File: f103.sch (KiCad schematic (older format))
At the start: 211 parts, among them J1 Conn_01x04_Female, J2 Conn_01x01_Male, J3 Conn_01x01_Male, J4 Conn_01x01_Male, Q1 2N7002, SW1 Rotary_Encoder_Switch, U1 STM32F103CBTx, U2 XC6206P332MR, U3 SRV05-4, Y1 8MHz

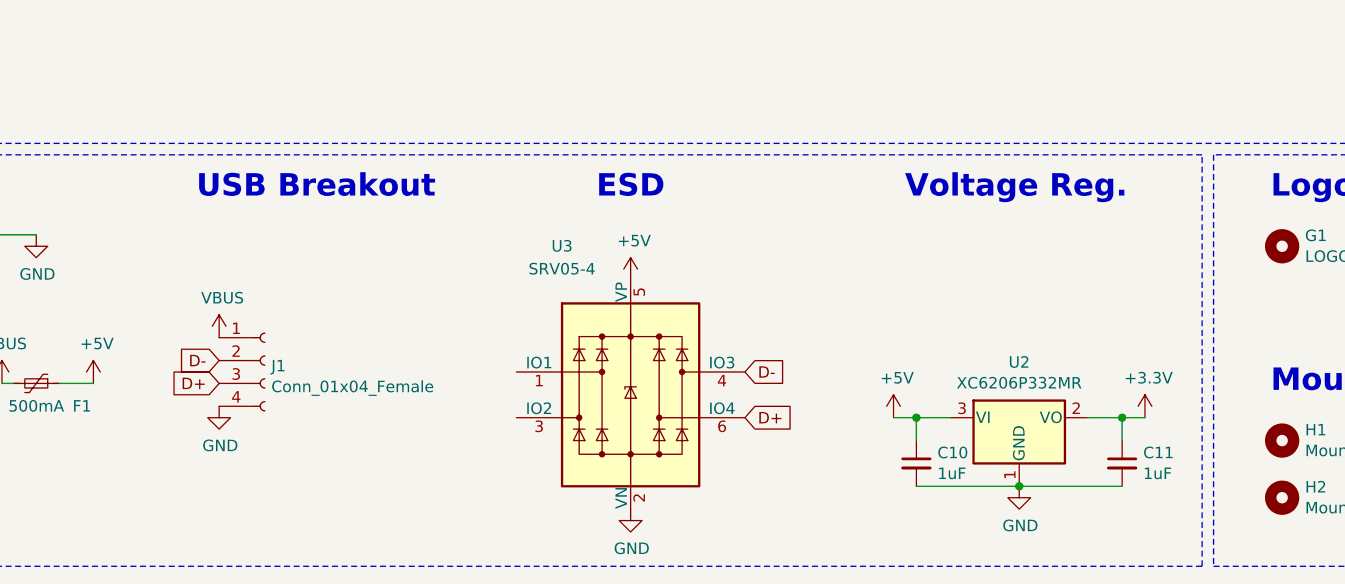
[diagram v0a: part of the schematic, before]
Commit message: DRC I
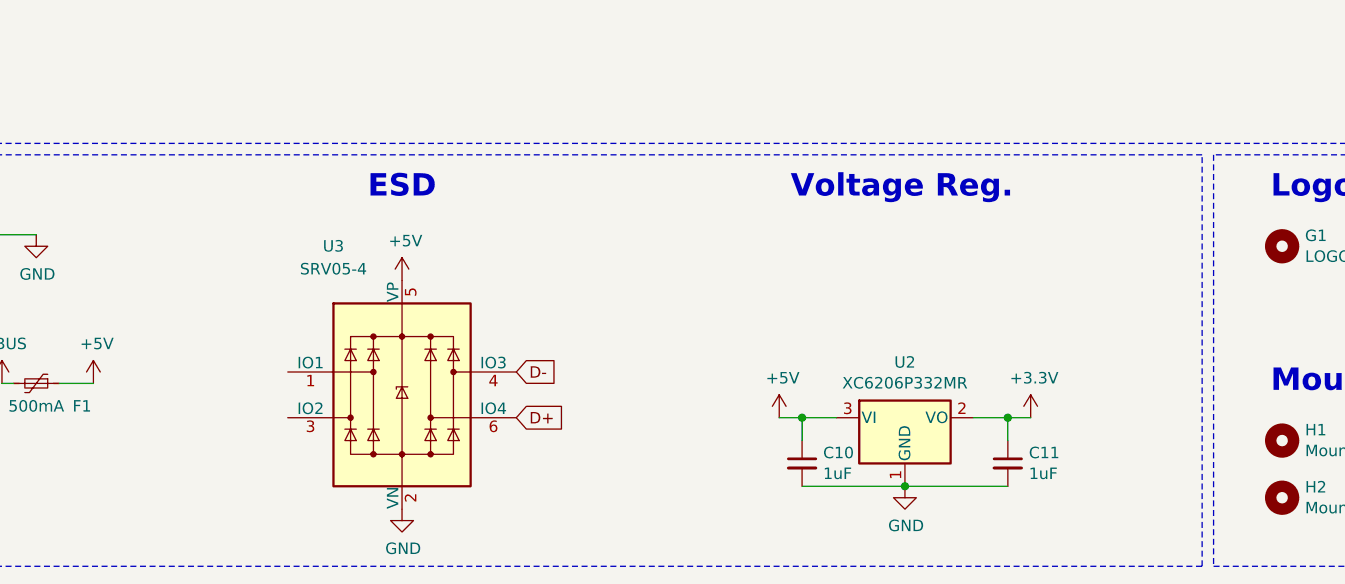
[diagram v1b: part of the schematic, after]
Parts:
- removed J1: Conn_01x04_Female, Connector_PinHeader_2.54mm:PinHeader_1x04_P2.54mm_Vertical, symbol Connector:Conn_01x04_Female
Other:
- note removed: "USB Breakout"
- moved on the sheet: C10, C11, U2, U3
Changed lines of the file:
@@
 EESchema Schematic File Version 4
+LIBS:f103-cache
 EELAYER 30 0
 EELAYER END
@@
 	1    0    0    -1
 $EndComp
-Text GLabel 5800 8050 2    50   Input ~ 0
+Text GLabel 4800 8050 2    50   Input ~ 0
 D-
 $Comp
 L power:+5V #PWR0116
 U 1 1 5FF47CBA
-P 5300 7650
-F 0 "#PWR0116" H 5300 7500 50  0001 C CNN
-F 1 "+5V" H 5315 7823 50  0000 C CNN
-F 2 "" H 5300 7650 50  0001 C CNN
-F 3 "" H 5300 7650 50  0001 C CNN
-	1    5300 7650
+P 4300 7650
+F 0 "#PWR0116" H 4300 7500 50  0001 C CNN
+F 1 "+5V" H 4315 7823 50  0000 C CNN
+F 2 "" H 4300 7650 50  0001 C CNN
+F 3 "" H 4300 7650 50  0001 C CNN
+	1    4300 7650
 	1    0    0    -1
 $EndComp
@@
 L power:GND #PWR0115
 U 1 1 5FF463F5
-P 5300 8650
-F 0 "#PWR0115" H 5300 8400 50  0001 C CNN
-F 1 "GND" H 5305 8477 50  0000 C CNN
-F 2 "" H 5300 8650 50  0001 C CNN
-F 3 "" H 5300 8650 50  0001 C CNN
-	1    5300 8650
+P 4300 8650
+F 0 "#PWR0115" H 4300 8400 50  0001 C CNN
+F 1 "GND" H 4305 8477 50  0000 C CNN
+F 2 "" H 4300 8650 50  0001 C CNN
+F 3 "" H 4300 8650 50  0001 C CNN
+	1    4300 8650
 	1    0    0    -1
 $EndComp
-Text GLabel 5800 8250 2    50   Input ~ 0
+Text GLabel 4800 8250 2    50   Input ~ 0
 D+
 $Comp
 L Power_Protection:SRV05-4 U3
 U 1 1 5FF42D8B
-P 5300 8150
-F 0 "U3" H 5000 8800 50  0000 C CNN
-F 1 "SRV05-4" H 5000 8700 50  0000 C CNN
-F 2 "Package_TO_SOT_SMD:SOT-23-6" H 6000 7700 50  0001 C CNN
-F 3 "http://www.onsemi.com/pub/Collateral/SRV05-4-D.PDF" H 5300 8150 50  0001 C CNN
-F 4 "C85364" H 5300 8150 50  0001 C CNN "Part #"
-	1    5300 8150
+P 4300 8150
+F 0 "U3" H 4000 8800 50  0000 C CNN
+F 1 "SRV05-4" H 4000 8700 50  0000 C CNN
+F 2 "Package_TO_SOT_SMD:SOT-23-6" H 5000 7700 50  0001 C CNN
+F 3 "http://www.onsemi.com/pub/Collateral/SRV05-4-D.PDF" H 4300 8150 50  0001 C CNN
+F 4 "C85364" H 4300 8150 50  0001 C CNN "Part #"
+	1    4300 8150
 	1    0    0    -1
 $EndComp
 Wire Wire Line
-	7450 8550 7000 8550
-Connection ~ 7000 8550
+	6950 8550 6500 8550
+Connection ~ 6500 8550
 Wire Wire Line
-	6550 8550 7000 8550
-Connection ~ 6550 8250
+	6050 8550 6500 8550
+Connection ~ 6050 8250
 Wire Wire Line
-	6550 8250 6450 8250
+	6050 8250 5950 8250
 Wire Wire Line
-	6550 8250 6550 8350
+	6050 8250 6050 8350
 Wire Wire Line
-	6700 8250 6550 8250
-Connection ~ 7450 8250
+	6200 8250 6050 8250
+Connection ~ 6950 8250
 Wire Wire Line
-	7450 8250 7550 8250
+	6950 8250 7050 8250
 Wire Wire Line
-	7450 8250 7450 8350
+	6950 8250 6950 8350
 Wire Wire Line
-	7300 8250 7450 8250
+	6800 8250 6950 8250
 $Comp
 L Device:C_Small C11
 U 1 1 5FF82A05
-P 7450 8450
-F 0 "C11" H 7542 8496 50  0000 L CNN
-F 1 "1uF" H 7542 8405 50  0000 L CNN
-F 2 "Capacitor_SMD:C_0603_1608Metric" H 7450 8450 50  0001 C CNN
-F 3 "~" H 7450 8450 50  0001 C CNN
-	1    7450 8450
+P 6950 8450
+F 0 "C11" H 7042 8496 50  0000 L CNN
+F 1 "1uF" H 7042 8405 50  0000 L CNN
+F 2 "Capacitor_SMD:C_0603_1608Metric" H 6950 8450 50  0001 C CNN
+F 3 "~" H 6950 8450 50  0001 C CNN
+	1    6950 8450
 	1    0    0    -1
 $EndComp
@@
 L Device:C_Small C10
 U 1 1 5FF81242
-P 6550 8450
-F 0 "C10" H 6642 8496 50  0000 L CNN
-F 1 "1uF" H 6642 8405 50  0000 L CNN
-F 2 "Capacitor_SMD:C_0603_1608Metric" H 6550 8450 50  0001 C CNN
-F 3 "~" H 6550 8450 50  0001 C CNN
-	1    6550 8450
+P 6050 8450
+F 0 "C10" H 6142 8496 50  0000 L CNN
+F 1 "1uF" H 6142 8405 50  0000 L CNN
+F 2 "Capacitor_SMD:C_0603_1608Metric" H 6050 8450 50  0001 C CNN
+F 3 "~" H 6050 8450 50  0001 C CNN
+	1    6050 8450
 	1    0    0    -1
 $EndComp
@@
 L power:GND #PWR0119
 U 1 1 5FF7FCD1
-P 7000 8550
-F 0 "#PWR0119" H 7000 8300 50  0001 C CNN
-F 1 "GND" H 7005 8377 50  0000 C CNN
-F 2 "" H 7000 8550 50  0001 C CNN
-F 3 "" H 7000 8550 50  0001 C CNN
-	1    7000 8550
+P 6500 8550
+F 0 "#PWR0119" H 6500 8300 50  0001 C CNN
+F 1 "GND" H 6505 8377 50  0000 C CNN
+F 2 "" H 6500 8550 50  0001 C CNN
+F 3 "" H 6500 8550 50  0001 C CNN
+	1    6500 8550
 	1    0    0    -1
 $EndComp
@@
 L power:+3.3V #PWR0118
 U 1 1 5FF7E7EA
-P 7550 8250
-F 0 "#PWR0118" H 7550 8100 50  0001 C CNN
-F 1 "+3.3V" H 7565 8423 50  0000 C CNN
-F 2 "" H 7550 8250 50  0001 C CNN
-F 3 "" H 7550 8250 50  0001 C CNN
-	1    7550 8250
+P 7050 8250
+F 0 "#PWR0118" H 7050 8100 50  0001 C CNN
+F 1 "+3.3V" H 7065 8423 50  0000 C CNN
+F 2 "" H 7050 8250 50  0001 C CNN
+F 3 "" H 7050 8250 50  0001 C CNN
+	1    7050 8250
 	1    0    0    -1
 $EndComp
@@
 L power:+5V #PWR0117
 U 1 1 5FF7D017
-P 6450 8250
-F 0 "#PWR0117" H 6450 8100 50  0001 C CNN
-F 1 "+5V" H 6465 8423 50  0000 C CNN
-F 2 "" H 6450 8250 50  0001 C CNN
-F 3 "" H 6450 8250 50  0001 C CNN
-	1    6450 8250
+P 5950 8250
+F 0 "#PWR0117" H 5950 8100 50  0001 C CNN
+F 1 "+5V" H 5965 8423 50  0000 C CNN
+F 2 "" H 5950 8250 50  0001 C CNN
+F 3 "" H 5950 8250 50  0001 C CNN
+	1    5950 8250
 	1    0    0    -1
 $EndComp
@@
 L Regulator_Linear:MCP1700-3302E_SOT23 U2
 U 1 1 5FF7B9AE
-P 7000 8250
-F 0 "U2" H 7000 8492 50  0000 C CNN
-F 1 "XC6206P332MR" H 7000 8401 50  0000 C CNN
-F 2 "Package_TO_SOT_SMD:SOT-23" H 7000 8475 50  0001 C CNN
-F 3 "http://ww1.microchip.com/downloads/en/DeviceDoc/20001826D.pdf" H 7000 8250 50  0001 C CNN
-F 4 "C5446" H 7000 8250 50  0001 C CNN "Part #"
-	1    7000 8250
+P 6500 8250
+F 0 "U2" H 6500 8492 50  0000 C CNN
+F 1 "XC6206P332MR" H 6500 8401 50  0000 C CNN
+F 2 "Package_TO_SOT_SMD:SOT-23" H 6500 8475 50  0001 C CNN
+F 3 "http://ww1.microchip.com/downloads/en/DeviceDoc/20001826D.pdf" H 6500 8250 50  0001 C CNN
+F 4 "C5446" H 6500 8250 50  0001 C CNN "Part #"
+	1    6500 8250
 	1    0    0    -1
 $EndComp
@@
 Text Notes 1950 7300 0    98   ~ 20
 USB
-Text Notes 6500 7300 0    98   ~ 20
+Text Notes 6000 7300 0    98   ~ 20
 Voltage Reg.
-Text Notes 5150 7300 0    98   ~ 20
+Text Notes 4150 7300 0    98   ~ 20
 ESD
 NoConn ~ 2050 8400
@@
 	1950 3900 2200 3900
 Connection ~ 2200 3900
-$Comp
-L power:VBUS #PWR0131
-U 1 1 60058240
-P 3500 7900
-F 0 "#PWR0131" H 3500 7750 50  0001 C CNN
-F 1 "VBUS" H 3515 8073 50  0000 C CNN
-F 2 "" H 3500 7900 50  0001 C CNN
-F 3 "" H 3500 7900 50  0001 C CNN
-	1    3500 7900
-	1    0    0    -1
-$EndComp
-$Comp
-L power:GND #PWR0132
-U 1 1 60057E3C
-P 3500 8200
-F 0 "#PWR0132" H 3500 7950 50  0001 C CNN
-F 1 "GND" H 3505 8027 50  0000 C CNN
-F 2 "" H 3500 8200 50  0001 C CNN
-F 3 "" H 3500 8200 50  0001 C CNN
-	1    3500 8200
-	1    0    0    -1
-$EndComp
-Text GLabel 3500 8100 0    50   Input ~ 0
-D+
-Text GLabel 3500 8000 0    50   Input ~ 0
-D-
-$Comp
-L Connector:Conn_01x04_Female J1
-U 1 1 60056004
-P 3700 8000
-F 0 "J1" H 3728 7976 50  0000 L CNN
-F 1 "Conn_01x04_Female" H 3728 7885 50  0000 L CNN
-F 2 "Connector_PinHeader_2.54mm:PinHeader_1x04_P2.54mm_Vertical" H 3700 8000 50  0001 C CNN
-F 3 "~" H 3700 8000 50  0001 C CNN
-	1    3700 8000
-	1    0    0    -1
-$EndComp
 Wire Notes Line
 	550  8900 7800 8900
-Text Notes 3400 7300 0    98   ~ 20
-USB Breakout
 $Comp
 L Device:Rotary_Encoder_Switch SW1
